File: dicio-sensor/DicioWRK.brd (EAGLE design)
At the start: 106.7 x 90.2 mm, 59 parts, among them J1 WTB-2, J2 WTB-2, J6 WTB-2, J7 TERM10, Q1 BSS84, Q2 BSS84, Q3 BSS84, Q4 BSS84, Q5 BSS84, U1 78MM6610+PSU, U2 APDS-9005, U3 MCP9700, U4 DK-1A-L2-3, U5 RAC01-3.3, U9 MCP3202SOIC

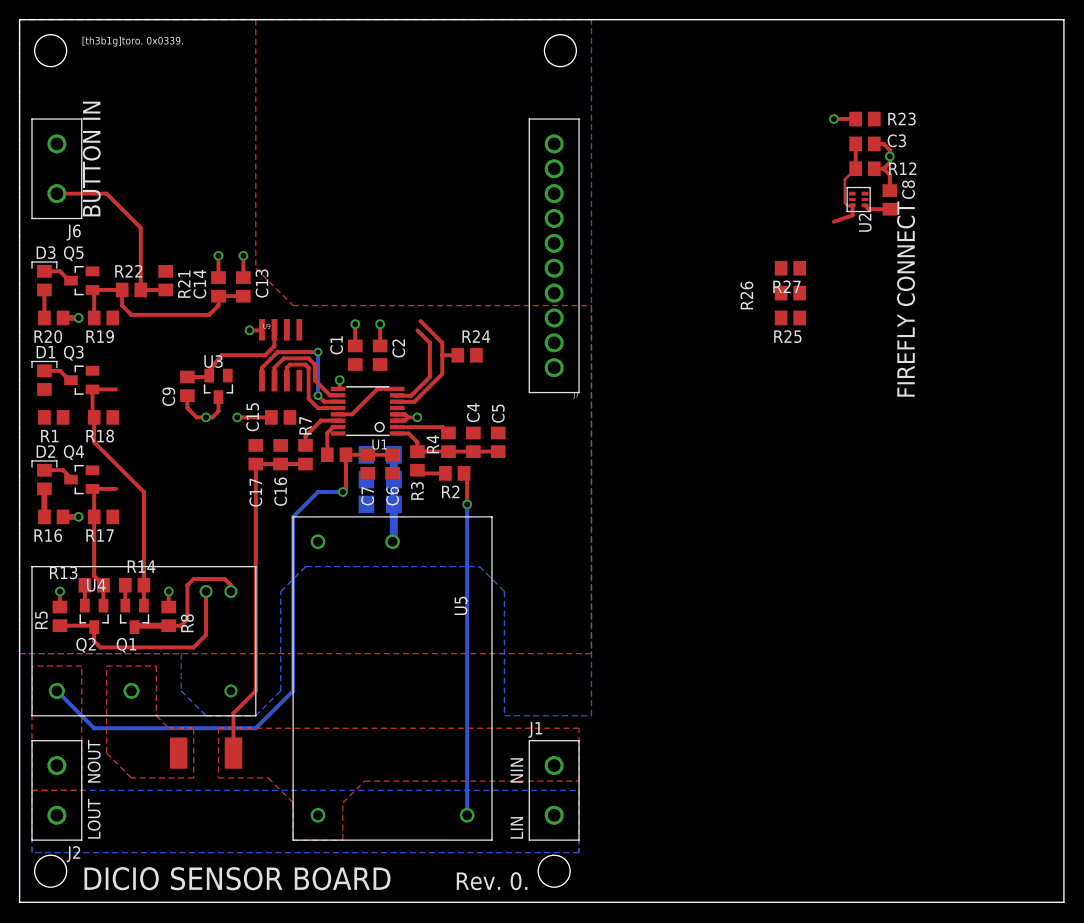
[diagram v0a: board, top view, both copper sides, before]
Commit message: Dicio sensor Rev 1
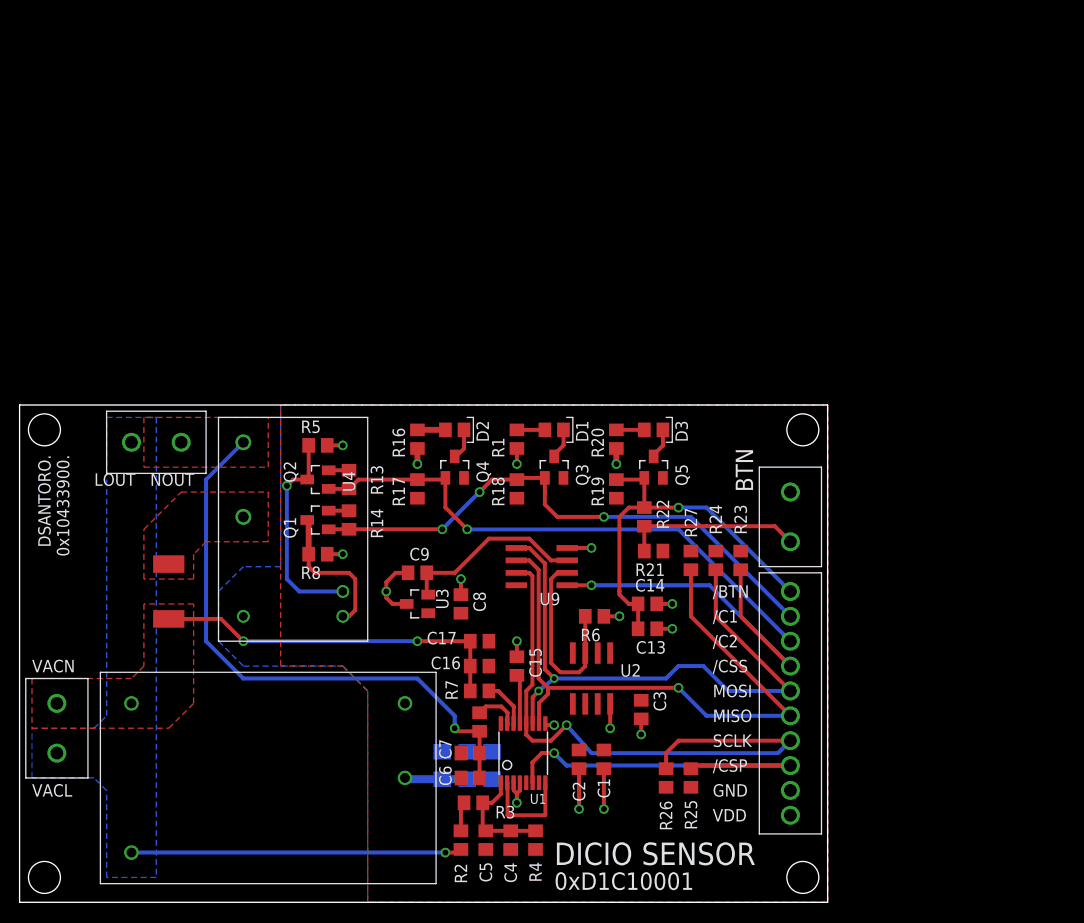
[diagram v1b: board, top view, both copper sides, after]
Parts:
- removed R12: 3.3k, resistor:R0805
- added R6: 10k, resistor:R0805
- U2: value APDS-9005 -> TSL250RD; device TORO:APDS-9005 -> TORO:SOIC8
- moved J6 82.9 mm to (78.7, 36.8)
- moved D3 64.1 mm to (64.8, 48.3), turned to 180 degrees
- moved C3 62.1 mm to (63.5, 19.7), turned to 270 degrees
- moved Q5 61.4 mm to (64.8, 44.5), turned to 0 degrees
- moved C8 60.2 mm to (45.1, 30.5)
- moved R20 58.8 mm to (61.0, 47.3), turned to 90 degrees
- moved R22 57.3 mm to (63.8, 39.4), turned to 90 degrees
- moved R21 57.0 mm to (64.8, 35.9), turned to 0 degrees
- moved U2 56.9 mm to (58.4, 22.9), turned to 0 degrees
- moved R19 55.2 mm to (61.0, 42.2), turned to 270 degrees
- moved C14 54.5 mm to (64.1, 30.5), turned to 0 degrees
- moved C13 54.1 mm to (64.1, 27.9), turned to 0 degrees
- moved D1 52.3 mm to (54.6, 48.3), turned to 180 degrees
- moved J7 51.7 mm to (78.7, 8.89)
- moved J1 51.2 mm to (3.81, 20.3)
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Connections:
- removed net !ALARM!: J7.P$2, U1.7
- removed net !FAULT!: J7.P$1, U1.5
- removed net S_LIGHT: C3.1, R12.2, U2.6, U9.2
- new net N$6: R6.2, U2.7, U9.2
- net !C1_EN!: now also J7.P$9; no longer J7.P$8
- net !C2_EN!: now also J7.P$8; no longer J7.P$9
- net !CS_PWR!: now also J7.P$3, R25.1; no longer J7.P$6, R24.1
- net GND: now also J7.P$2, R6.1, U2.4; no longer R12.1
- net MISO: now also J7.P$5, R27.1; no longer J7.P$4, R26.1
- net MOSI: now also J7.P$6, R24.1; no longer J7.P$5, R27.1
- net SCLK: now also J7.P$4, R26.1; no longer J7.P$3, R25.1
- net VDD: now also C3.1, J7.P$1, U2.6; no longer U2.1
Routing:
- net MISO: track 10.7 -> 64.2 mm, vias 0 -> 1
- net SCLK: track 10.4 -> 62.8 mm, vias 0 -> 1
- net MOSI: track 14.4 -> 62.6 mm
- net !C2_EN!: track 14.8 -> 56.3 mm, vias 0 -> 1
- net !CS_SENSE!: track 0.00 -> 38.2 mm, vias 0 -> 1
- net !C1_EN!: track 27.5 -> 57.7 mm, vias 0 -> 3
- net !CS_PWR!: track 13.7 -> 39.8 mm, vias 0 -> 1
- net N$6: track 0.00 -> 19.7 mm
- net !BUTTON!: track 21.9 -> 40.4 mm, vias 0 -> 1
- net S_LIGHT: track 10.5 -> 0.00 mm
- net !ALARM!: track 9.84 -> 0.00 mm
- net S_TEMP: track 12.2 -> 19.0 mm
- net GND: track 39.5 -> 42.7 mm, vias 14 -> 18
- net N$10: track 0.00 -> 2.86 mm
- net VDD: track 30.6 -> 28.6 mm, vias 1 -> 0
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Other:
- board size 106.7 x 90.2 mm -> 82.5 x 50.8 mm
- board text added: "/BTN"
- board text added: "/C1"
- board text added: "/C2"
- board text added: "/CSP"
- board text added: "/CSS"
- board text added: "0xD1C10001"
- board text added: "BTN"
- board text added: "DICIO SENSOR"
- board text added: "DSANTORO. 0x10433900."
- board text added: "GND"
- board text added: "MISO"
- board text added: "MOSI"
- board text added: "SCLK"
- board text added: "VACL"
- board text added: "VACN"
- board text added: "VDD"
- board text removed: "BUTTON IN"
- board text removed: "DICIO SENSOR BOARD"
- board text removed: "FIREFLY CONNECT"
- board text removed: "LIN"
- board text removed: "NIN"
- board text removed: "Rev. 0."
- board text removed: "[th3b1g]toro. 0x0339."
